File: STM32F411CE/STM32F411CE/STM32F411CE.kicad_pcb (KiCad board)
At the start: 2 copper layers, 27.9 x 48.5 mm, 16 parts, among them J1 USB_B_Mini, J2 Conn_01x19_Male, J3 Conn_01x19_Male, U2 USBLC6-2SC6, U3 STM32F411CEUx, Y1 Crystal_GND24

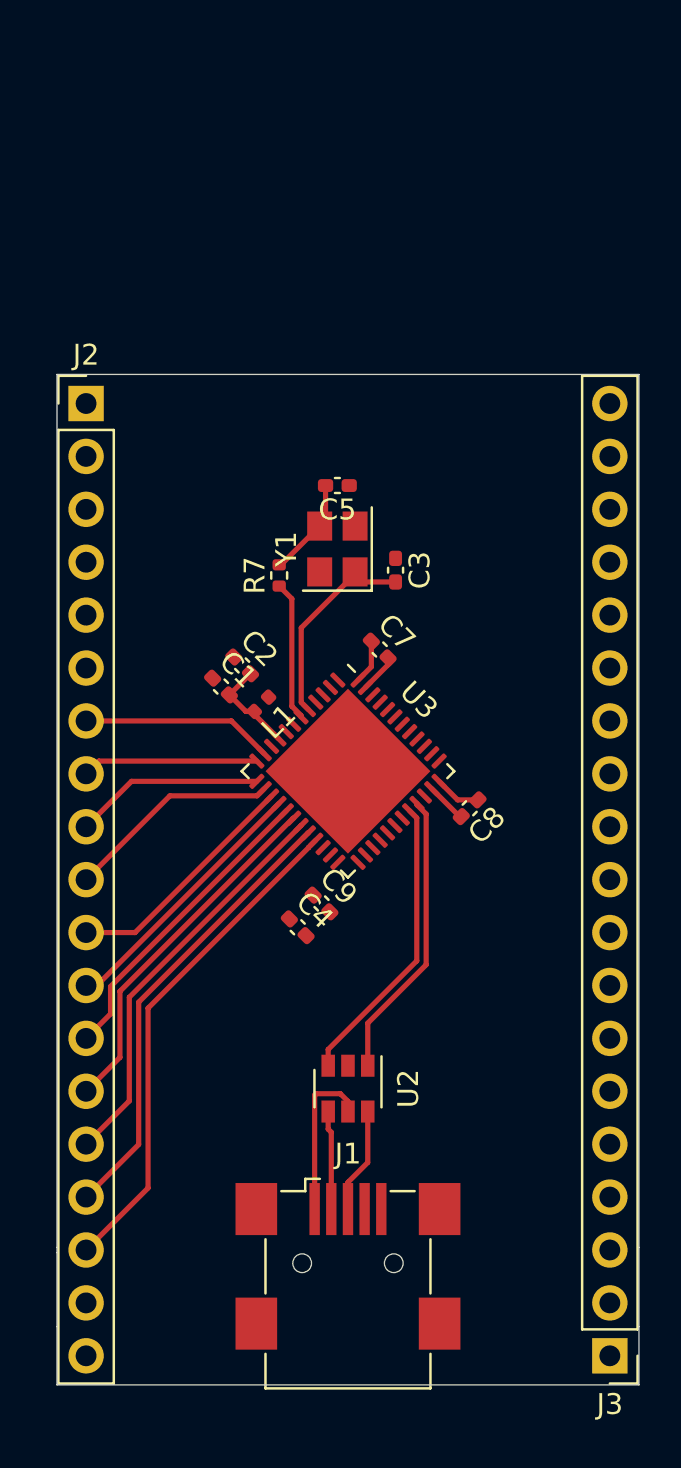
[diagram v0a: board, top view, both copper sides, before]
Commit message: do most of the breakout
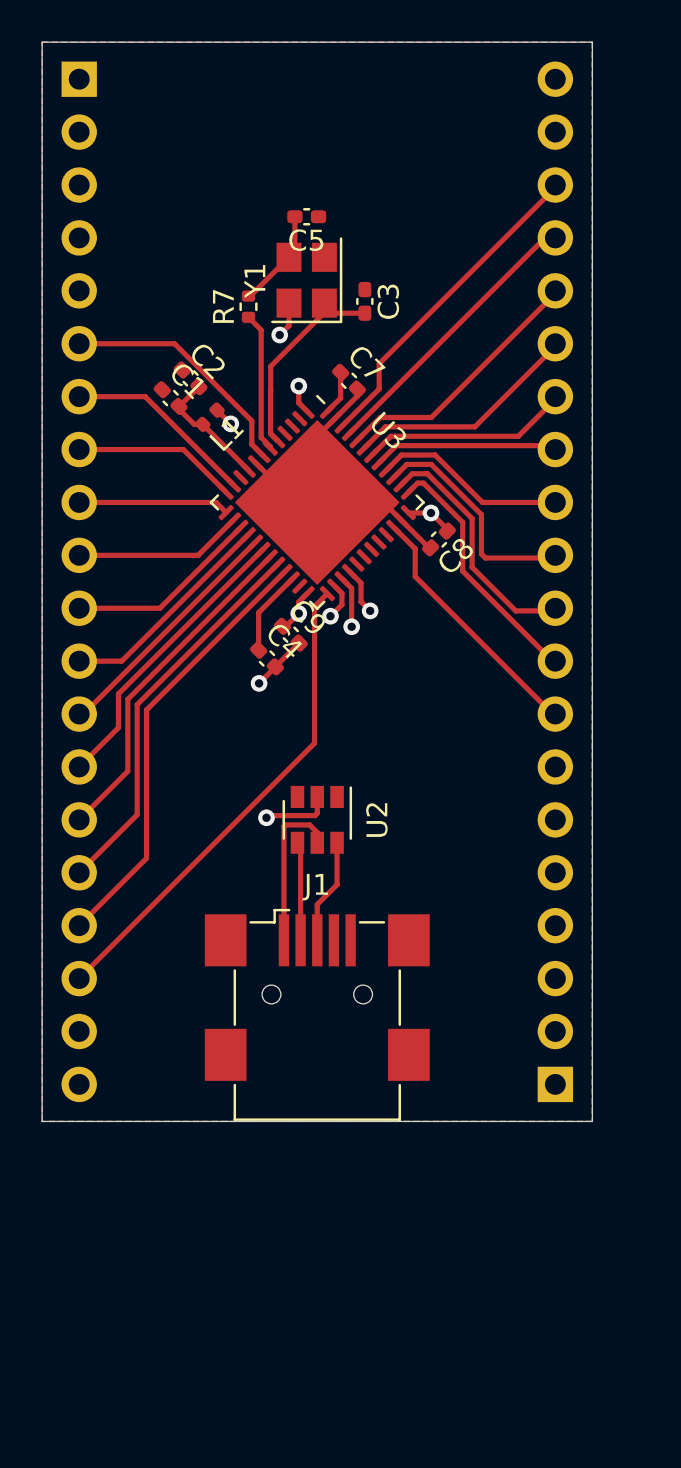
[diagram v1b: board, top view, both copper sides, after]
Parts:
- J2, J3: value Conn_01x19_Male -> Conn_01x20_Male; footprint Connector_PinHeader_2.54mm:PinHeader_1x19_P2.54mm_Vertical -> Connector_PinHeader_2.54mm:PinHeader_1x20_P2.54mm_Vertical; moved to B.Cu
- moved J2 15.6 mm to (13.8, 13.8), turned to 180 degrees
- moved C1 14.1 mm to (18.2, 29.1)
- moved L1 14.0 mm to (20.0, 30.0)
- moved C2 14.0 mm to (19.1, 28.1)
- moved J3 13.3 mm to (36.6, 62.0), turned to 0 degrees
- moved C9 13.0 mm to (23.9, 40.4)
- moved U3 13.0 mm to (25.2, 34.1)
- moved C3 13.0 mm to (27.5, 24.4)
- moved C5 13.0 mm to (24.7, 20.4)
- moved C7 13.0 mm to (26.7, 28.2)
- moved Y1 13.0 mm to (24.7, 23.4)
- moved C4 13.0 mm to (22.8, 41.6)
- moved C8 13.0 mm to (31.0, 35.9)
- moved J1 13.0 mm to (25.2, 57.7)
- moved R7 13.0 mm to (21.9, 24.7)
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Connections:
- J2 pad 19: +5V -> GND
- J2 pad 3: PC13 -> (no net)
- J2 pad 4: PC14 -> (no net)
- J2 pad 5: ~RST -> (no net)
- J2 pad 6: PC15 -> ~RST
- J3 pad 5: PA8 -> (no net)
- J3 pad 6: PA9 -> (no net)
- J3 pad 7: PA10 -> (no net)
- U3 pad 2: PC13 -> (no net)
- U3 pad 29: PA8 -> (no net)
- U3 pad 3: PC14 -> (no net)
- U3 pad 30: PA9 -> (no net)
- U3 pad 31: PA10 -> (no net)
- U3 pad 4: PC15 -> (no net)
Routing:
- net PB13: track 0.00 -> 26.2 mm, vias 0 -> 1
- net PB14: track 0.00 -> 23.4 mm, vias 0 -> 1
- net PB12: track 0.00 -> 23.4 mm
- net PB15: track 0.00 -> 21.1 mm, vias 0 -> 1
- net +BATT: track 0.00 -> 20.5 mm, vias 0 -> 1
- net GND: track 3.84 -> 24.1 mm, vias 0 -> 3
- net PB9: track 0.00 -> 15.7 mm
- net USB_D-: track 14.1 -> 0.00 mm
- net USB_D+: track 13.9 -> 0.00 mm
- net PB8: track 0.00 -> 13.7 mm
- net BOOT0: track 0.00 -> 12.5 mm
- net SWDIO: track 0.00 -> 12.3 mm
- net SWDCLK: track 0.00 -> 12.2 mm
- net PA15: track 0.00 -> 11.7 mm
- net ~RST: track 0.00 -> 11.7 mm
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- added copper zone on In2.Cu, net +3V3
- added copper zone on B.Cu, net GND
- added copper zone on F.Cu, net GND
- added copper zone on In1.Cu, net GND
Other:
- board size 27.9 x 48.5 mm -> 26.4 x 51.8 mm
- copper layers 2 -> 4
